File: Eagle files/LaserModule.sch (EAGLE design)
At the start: 6 parts, among them Q1 IRF510

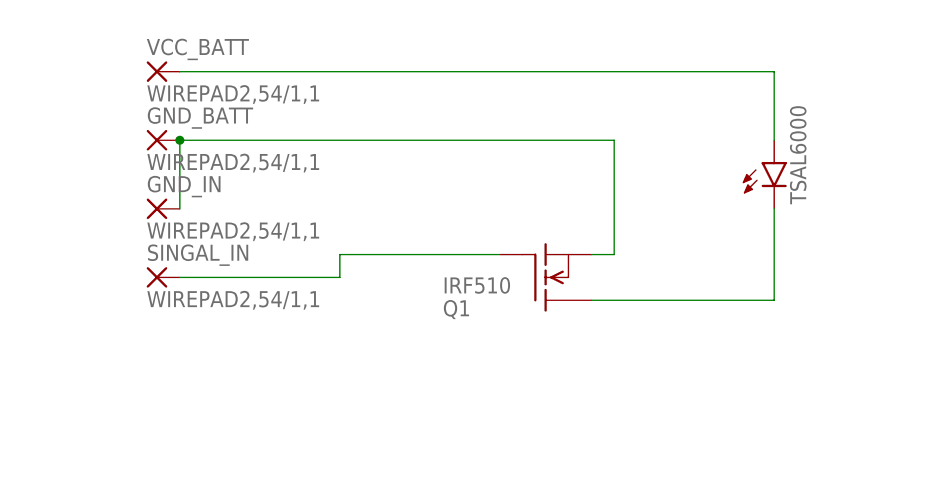
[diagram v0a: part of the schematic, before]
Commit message: New Lazer
Changed some stuff in the laser module, nbd.
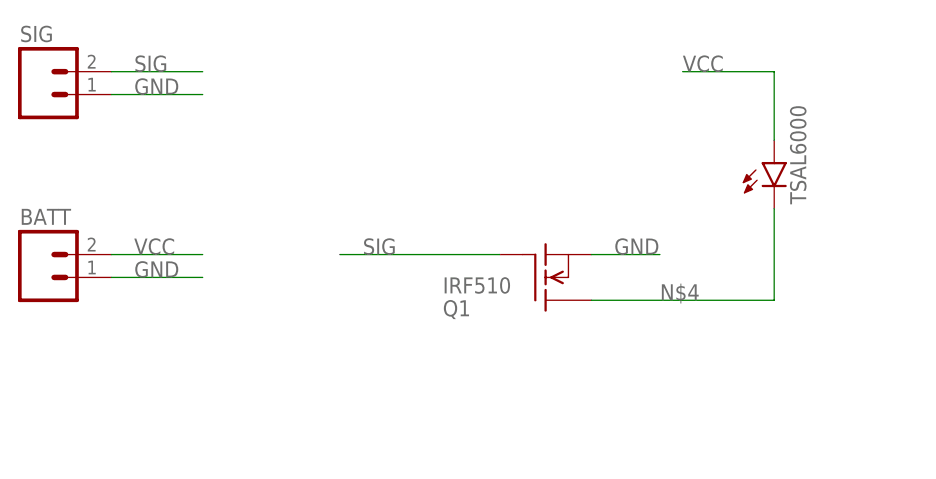
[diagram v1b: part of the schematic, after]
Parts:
- removed GND_BATT, GND_IN, SINGAL_IN, VCC_BATT: WIREPAD2,54/1,1, wirepad:WIREPAD2,54/1,1
- added BATT, SIG: (no value), SparkFun-Connectors:M02PTH
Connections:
- removed net N$1: Q1.G, SINGAL_IN.P
- removed net N$3: TSAL6000.A, VCC_BATT.P
- new net SIG: Q1.G, SIG.2
- new net VCC: BATT.2, TSAL6000.A
- net GND: now also BATT.1, SIG.1; no longer GND_BATT.P, GND_IN.P
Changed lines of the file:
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@@
 <layer number="112" name="tSilk" color="7" fill="1" visible="yes" active="yes"/>
 <layer number="113" name="IDFDebug" color="4" fill="1" visible="yes" active="yes"/>
+<layer number="114" name="Badge_Outline" color="7" fill="1" visible="yes" active="yes"/>
+<layer number="115" name="ReferenceISLANDS" color="7" fill="1" visible="yes" active="yes"/>
 <layer number="116" name="Patch_BOT" color="9" fill="4" visible="yes" active="yes"/>
 <layer number="118" name="Rect_Pads" color="7" fill="1" visible="yes" active="yes"/>
@@
 <parts>
 <part name="Q1" library="transistor-fet" deviceset="IRF510" device=""/>
-<part name="VCC_BATT" library="wirepad" deviceset="WIREPAD" device="2,54/1,1"/>
-<part name="GND_BATT" library="wirepad" deviceset="WIREPAD" device="2,54/1,1"/>
-<part name="GND_IN" library="wirepad" deviceset="WIREPAD" device="2,54/1,1"/>
-<part name="SINGAL_IN" library="wirepad" deviceset="WIREPAD" device="2,54/1,1" value="WIREPAD2,54/1,1"/>
 <part name="TSAL6000" library="SparkFun-LED" deviceset="LED" device="5MM"/>
 <part name="FRAME1" library="frames" deviceset="LETTER_L" device=""/>
+<part name="SIG" library="SparkFun-Connectors" deviceset="M02" device="PTH"/>
+<part name="BATT" library="SparkFun-Connectors" deviceset="M02" device="PTH"/>
 </parts>
 <sheets>
@@
 <instances>
 <instance part="Q1" gate="G$1" x="53.34" y="38.1" rot="MR180"/>
-<instance part="VCC_BATT" gate="G$1" x="10.16" y="60.96"/>
-<instance part="GND_BATT" gate="G$1" x="10.16" y="53.34"/>
-<instance part="GND_IN" gate="G$1" x="10.16" y="45.72"/>
-<instance part="SINGAL_IN" gate="G$1" x="10.16" y="38.1"/>
 <instance part="TSAL6000" gate="G$1" x="78.74" y="50.8"/>
 <instance part="FRAME1" gate="G$1" x="-68.58" y="-53.34"/>
 <instance part="FRAME1" gate="G$2" x="78.74" y="-53.34"/>
+<instance part="SIG" gate="G$1" x="-2.54" y="58.42"/>
+<instance part="BATT" gate="G$1" x="-2.54" y="38.1"/>
 </instances>
 <busses>
 </busses>
 <nets>
-<net name="N$1" class="0">
-<segment>
-<pinref part="SINGAL_IN" gate="G$1" pin="P"/>
-<pinref part="Q1" gate="G$1" pin="G"/>
-<wire x1="12.7" y1="38.1" x2="30.48" y2="38.1" width="0.1524" layer="91"/>
-<wire x1="30.48" y1="38.1" x2="30.48" y2="40.64" width="0.1524" layer="91"/>
-<wire x1="30.48" y1="40.64" x2="48.26" y2="40.64" width="0.1524" layer="91"/>
-</segment>
-</net>
 <net name="GND" class="0">
 <segment>
 <pinref part="Q1" gate="G$1" pin="S"/>
-<wire x1="58.42" y1="40.64" x2="60.96" y2="40.64" width="0.1524" layer="91"/>
-<wire x1="60.96" y1="40.64" x2="60.96" y2="53.34" width="0.1524" layer="91"/>
-<wire x1="60.96" y1="53.34" x2="12.7" y2="53.34" width="0.1524" layer="91"/>
-<pinref part="GND_BATT" gate="G$1" pin="P"/>
-<pinref part="GND_IN" gate="G$1" pin="P"/>
-<wire x1="12.7" y1="53.34" x2="12.7" y2="45.72" width="0.1524" layer="91"/>
-<junction x="12.7" y="53.34"/>
+<wire x1="58.42" y1="40.64" x2="66.04" y2="40.64" width="0.1524" layer="91"/>
+<label x="60.96" y="40.64" size="1.778" layer="95"/>
 </segment>
-</net>
-<net name="N$3" class="0">
 <segment>
-<pinref part="VCC_BATT" gate="G$1" pin="P"/>
-<pinref part="TSAL6000" gate="G$1" pin="A"/>
-<wire x1="12.7" y1="60.96" x2="78.74" y2="60.96" width="0.1524" layer="91"/>
-<wire x1="78.74" y1="60.96" x2="78.74" y2="53.34" width="0.1524" layer="91"/>
+<pinref part="SIG" gate="G$1" pin="1"/>
+<wire x1="15.24" y1="58.42" x2="5.08" y2="58.42" width="0.1524" layer="91"/>
+<label x="7.62" y="58.42" size="1.778" layer="95"/>
+</segment>
+<segment>
+<pinref part="BATT" gate="G$1" pin="1"/>
+<wire x1="15.24" y1="38.1" x2="5.08" y2="38.1" width="0.1524" layer="91"/>
+<label x="7.62" y="38.1" size="1.778" layer="95"/>
 </segment>
 </net>
@@
 <wire x1="58.42" y1="35.56" x2="78.74" y2="35.56" width="0.1524" layer="91"/>
 <wire x1="78.74" y1="35.56" x2="78.74" y2="45.72" width="0.1524" layer="91"/>
+<label x="66.04" y="35.56" size="1.778" layer="95"/>
 </segment>
 </net>
+<net name="SIG" class="0">
+<segment>
+<pinref part="SIG" gate="G$1" pin="2"/>
+<wire x1="15.24" y1="60.96" x2="5.08" y2="60.96" width="0.1524" layer="91"/>
+<label x="7.62" y="60.96" size="1.778" layer="95"/>
+</segment>
+<segment>
+<pinref part="Q1" gate="G$1" pin="G"/>
+<wire x1="30.48" y1="40.64" x2="48.26" y2="40.64" width="0.1524" layer="91"/>
+<label x="33.02" y="40.64" size="1.778" layer="95"/>
+</segment>
+</net>
+<net name="VCC" class="0">
+<segment>
+<pinref part="BATT" gate="G$1" pin="2"/>
+<wire x1="15.24" y1="40.64" x2="5.08" y2="40.64" width="0.1524" layer="91"/>
+<label x="7.62" y="40.64" size="1.778" layer="95"/>
+</segment>
+<segment>
+<pinref part="TSAL6000" gate="G$1" pin="A"/>
+<wire x1="68.58" y1="60.96" x2="78.74" y2="60.96" width="0.1524" layer="91"/>
+<wire x1="78.74" y1="60.96" x2="78.74" y2="53.34" width="0.1524" layer="91"/>
+<label x="68.58" y="60.96" size="1.778" layer="95"/>
+</segment>
+</net>
